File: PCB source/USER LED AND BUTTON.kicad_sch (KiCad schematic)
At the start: 7 parts

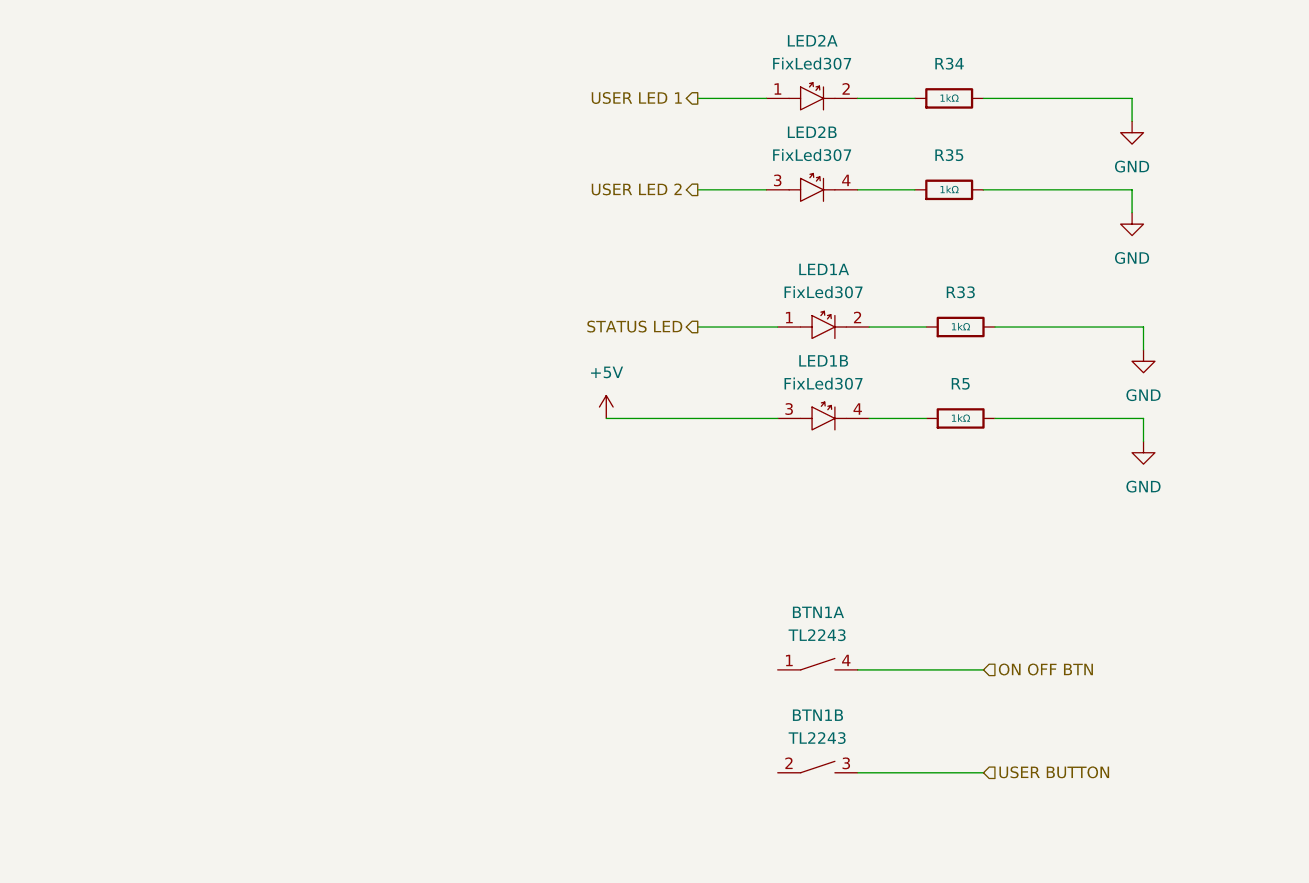
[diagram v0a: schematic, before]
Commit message: Pass ERC
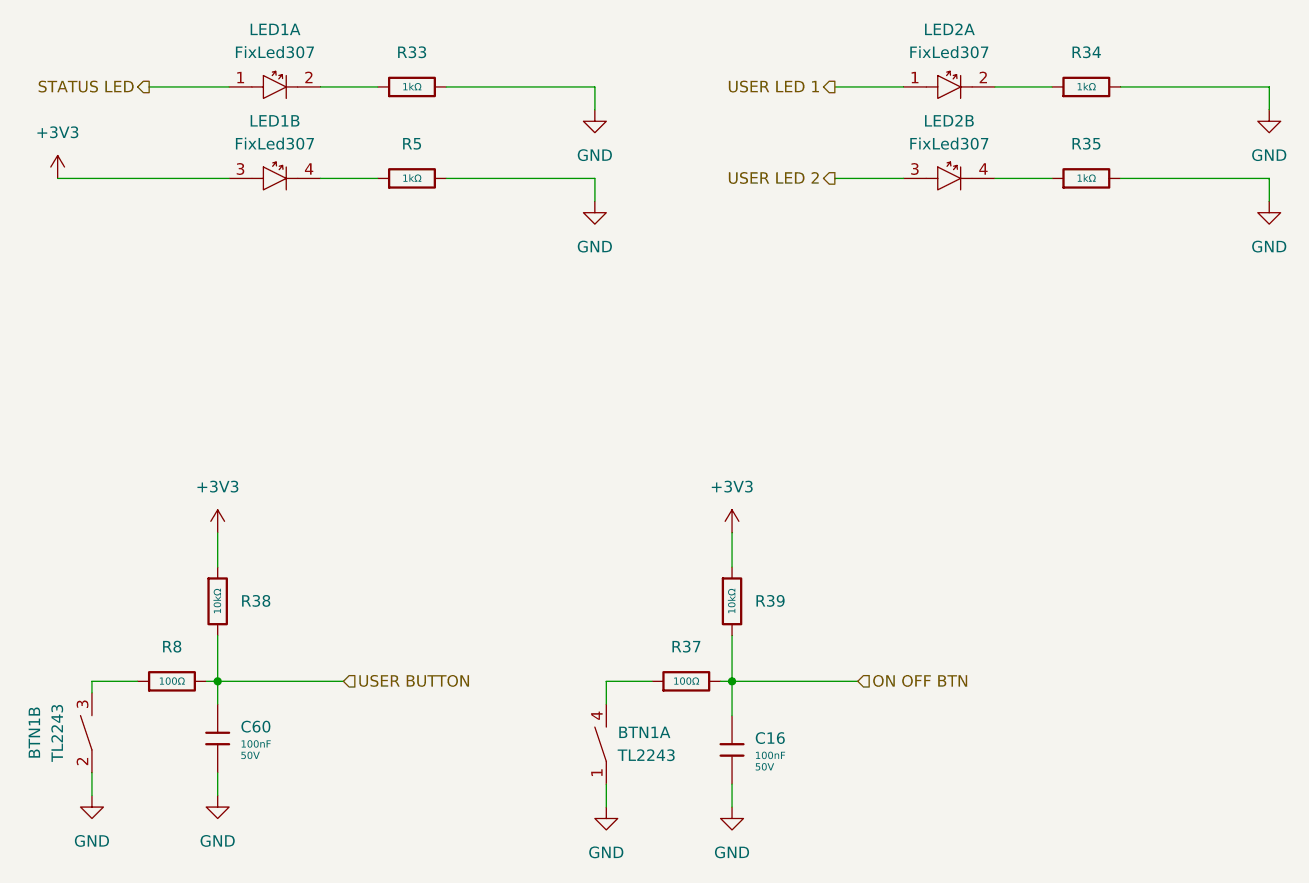
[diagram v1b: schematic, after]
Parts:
- added C16, C60: 100nF, PCM_JLCPCB:C_0402, symbol PCM_JLCPCB-Capacitors:0402,100nF,(2)
- added R37, R8: 100Ω, PCM_JLCPCB:R_0402, symbol PCM_JLCPCB-Resistors:0402,100Ω
- added R38, R39: 10kΩ, PCM_JLCPCB:R_0402, symbol PCM_JLCPCB-Resistors:0402,10kΩ
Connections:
- net GND: now also BTN1.1, BTN1.2, C16.2, C60.2
- net ON OFF BTN: now also C16.1, R37.2, R39.2; no longer BTN1.4
- net USER BUTTON: now also C60.1, R38.2, R8.2; no longer BTN1.3
- net +5V renamed +3V3
- net +3V3: now also R38.1, R39.1
- new net: BTN1.4, R37.1
- new net: BTN1.3, R8.1
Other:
- moved on the sheet: BTN1A, BTN1B, LED1A, LED1B, LED2A, LED2B, R33, R34, R35, R5
